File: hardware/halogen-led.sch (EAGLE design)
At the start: 33 parts

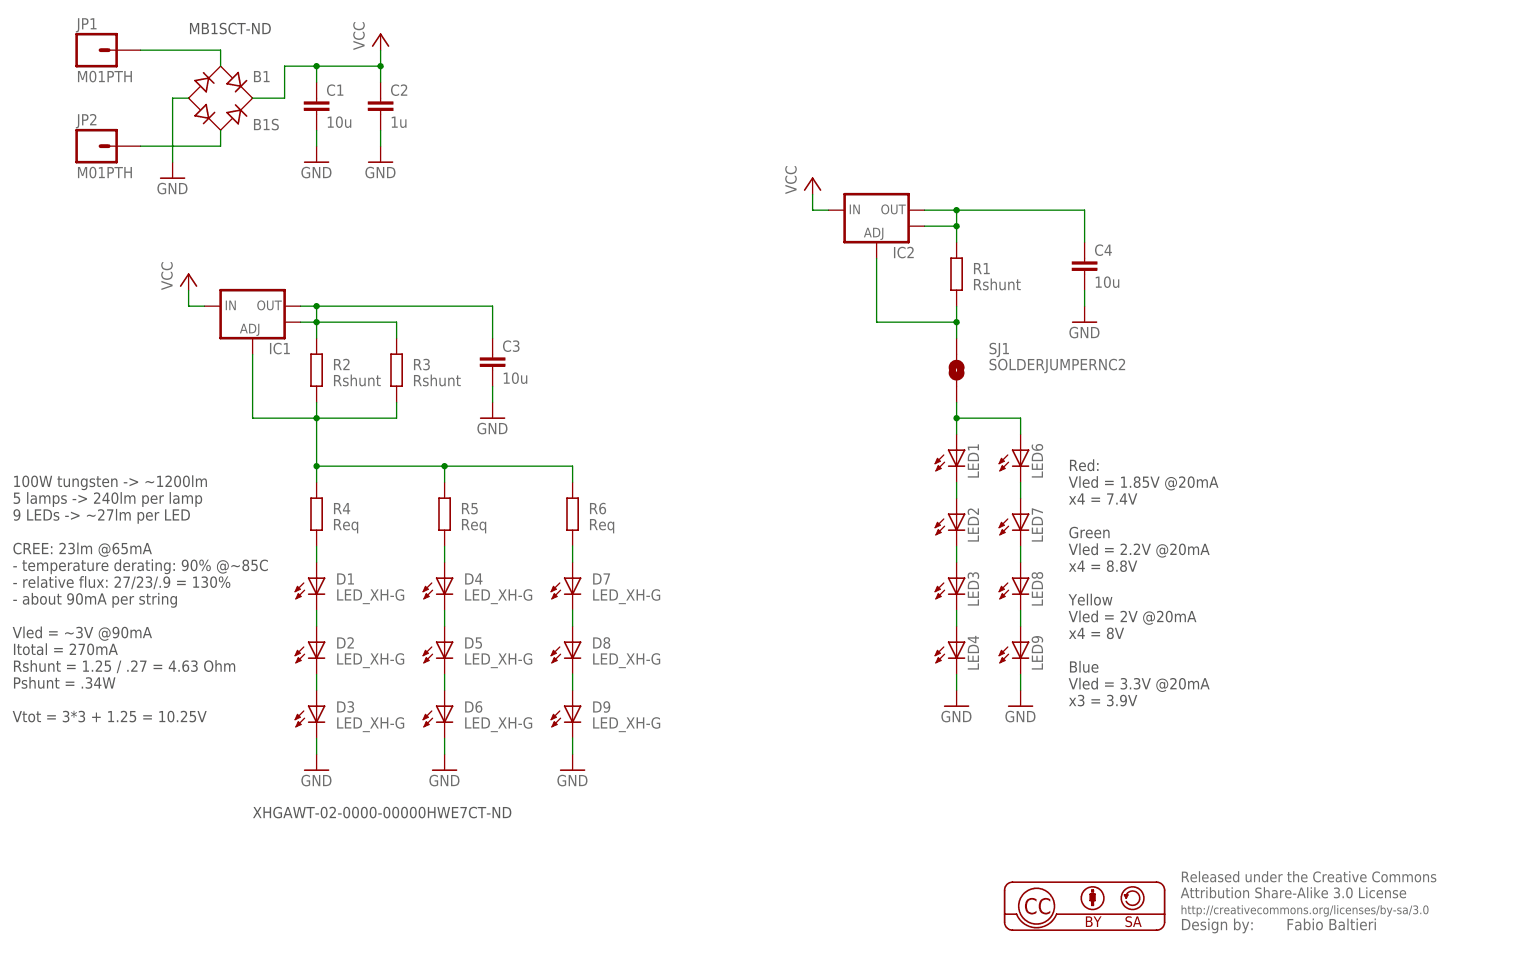
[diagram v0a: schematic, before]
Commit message: rc2
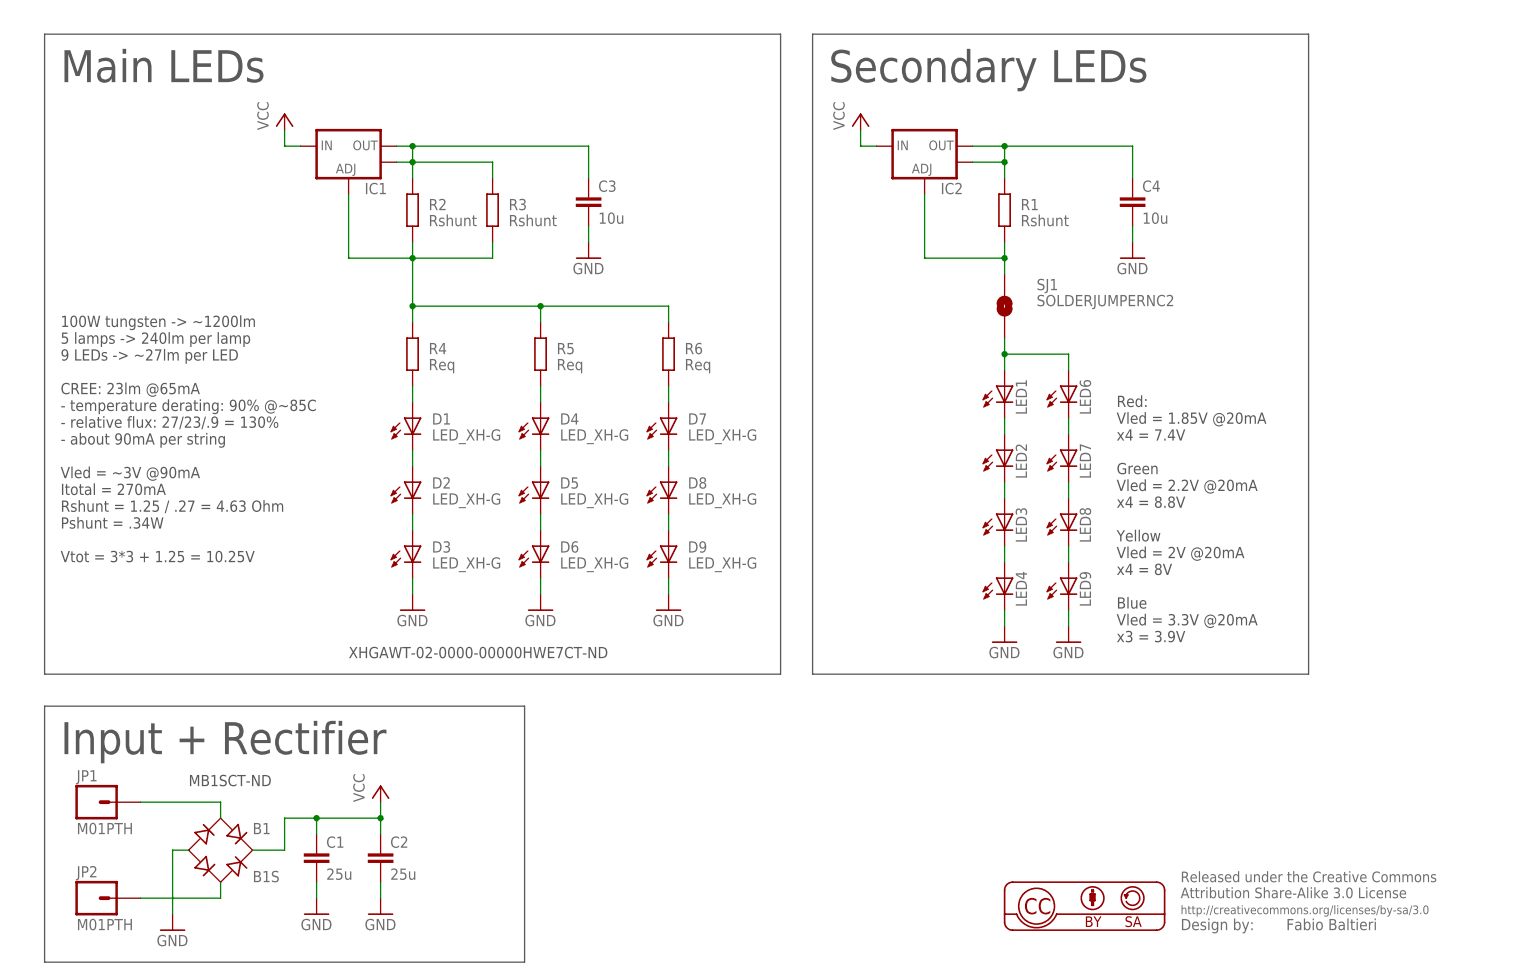
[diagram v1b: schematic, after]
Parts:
- C1: value 10u -> 25u
- C2: value 1u -> 25u
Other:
- note added: "Input + Rectifier"
- note added: "Main LEDs"
- note added: "Secondary LEDs"
- moved on the sheet: B1, C1, C2, C3, C4, D1, D2, D3, D4, D5, D6, D7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
